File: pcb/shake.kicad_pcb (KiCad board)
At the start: 2 copper layers, 22.4 x 41.9 mm, 15 parts, among them T1 TO-92L_Inline

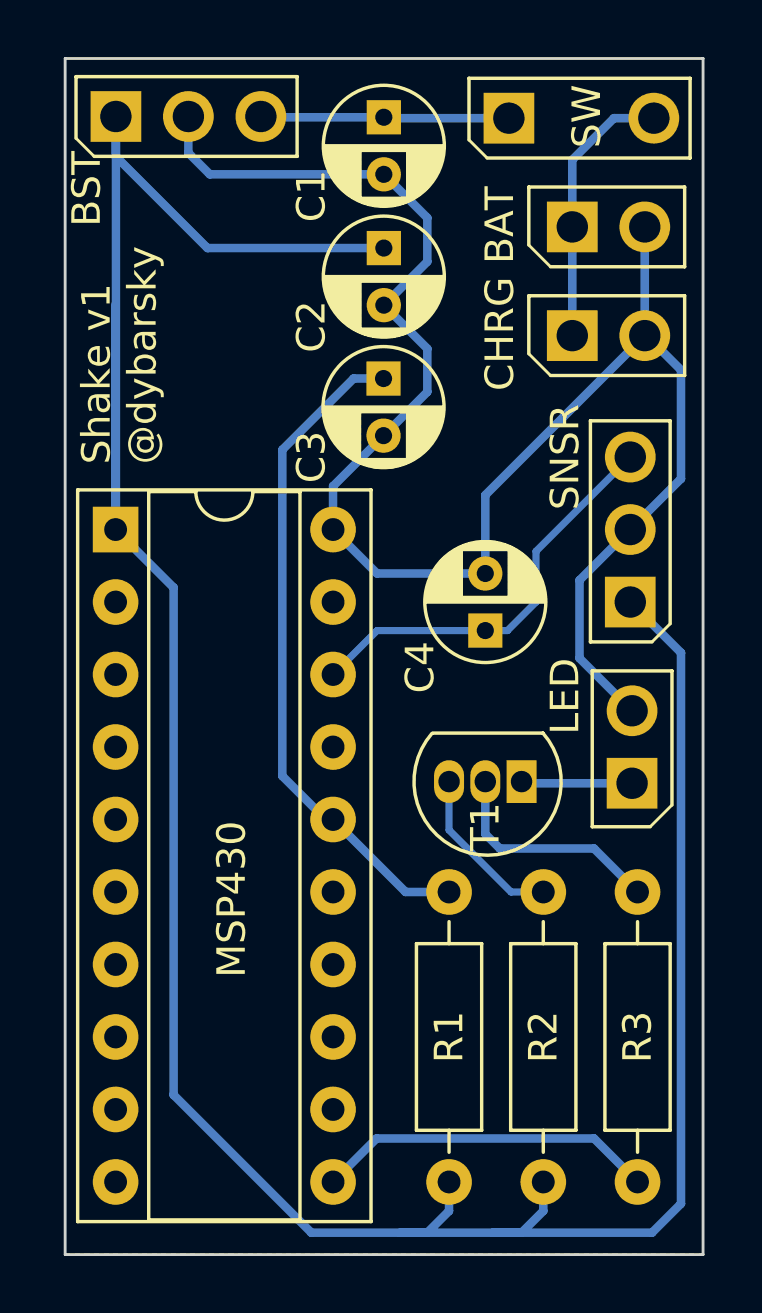
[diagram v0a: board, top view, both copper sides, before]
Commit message: Update kicad project
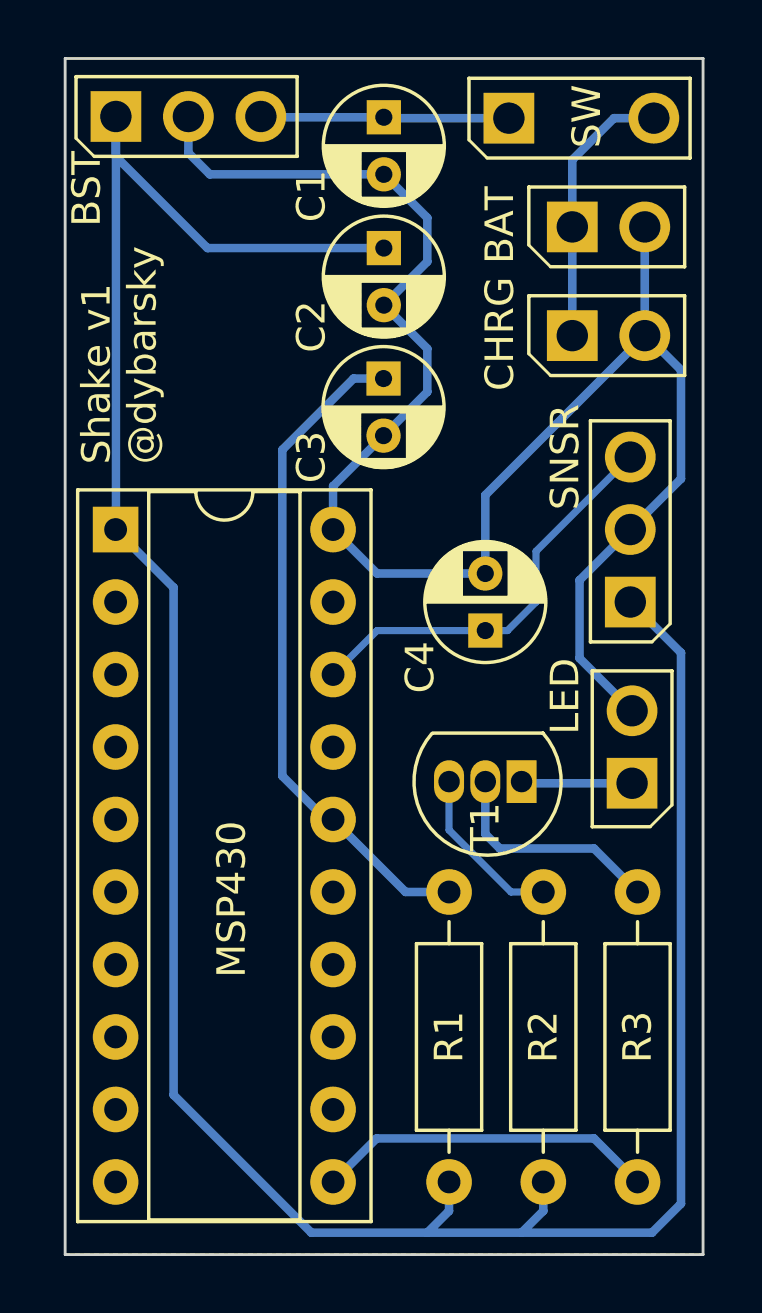
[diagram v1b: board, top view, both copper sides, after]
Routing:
- net +5V: track 110.5 -> 93.8 mm
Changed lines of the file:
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@@
     (grid_origin 85.08 69.591)
     (pcbplotparams
-      (layerselection 0x00010fc_ffffffff)
+      (layerselection 0x0001000_fffffffe)
       (plot_on_all_layers_selection 0x0000000_00000000)
       (disableapertmacros false)
@@
       (sketchpadsonfab false)
       (subtractmaskfromsilk false)
-      (outputformat 1)
+      (outputformat 5)
       (mirror false)
-      (drillshape 1)
+      (drillshape 2)
       (scaleselection 1)
       (outputdirectory "")
@@
   (segment (start 74.92 65.527) (end 74.92 61.717) (width 0.3) (layer "B.Cu") (net 3))
   (segment (start 55.118 67.564) (end 55.372 67.818) (width 0.3) (layer "F.Cu") (net 4))
-  (segment (start 55.108 59.431) (end 55.108 67.305) (width 0.3) (layer "B.Cu") (net 4))
   (segment (start 58.326401 57.442401) (end 55.118 54.234) (width 0.3) (layer "B.Cu") (net 4))
   (segment (start 55.118 52.832) (end 55.118 67.295) (width 0.3) (layer "B.Cu") (net 4))
   (segment (start 55.118 67.295) (end 55.108 67.305) (width 0.3) (layer "B.Cu") (net 4))
   (segment (start 73.904 91.943) (end 61.966 91.943) (width 0.3) (layer "B.Cu") (net 4))
-  (segment (start 69.332 91.943) (end 68.316 91.943) (width 0.3) (layer "B.Cu") (net 4))
-  (segment (start 66.03 91.943) (end 65.0775 91.943) (width 0.3) (layer "B.Cu") (net 4))
   (segment (start 64.506 57.442401) (end 58.326401 57.442401) (width 0.3) (layer "B.Cu") (net 4))
   (segment (start 57.14 87.117) (end 57.14 69.337) (width 0.3) (layer "B.Cu") (net 4))
@@
   (segment (start 66.792 91.181) (end 66.03 91.943) (width 0.3) (layer "B.Cu") (net 4))
   (segment (start 55.118 54.234) (end 55.118 52.832) (width 0.3) (layer "B.Cu") (net 4))
-  (segment (start 55.108 60.447) (end 55.108 67.305) (width 0.3) (layer "B.Cu") (net 4))
   (segment (start 70.094 90.165) (end 70.094 91.181) (width 0.3) (layer "B.Cu") (net 4))
   (segment (start 73.142 69.845) (end 74.92 71.623) (width 0.3) (layer "B.Cu") (net 4))

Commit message: Update pcb and schematics
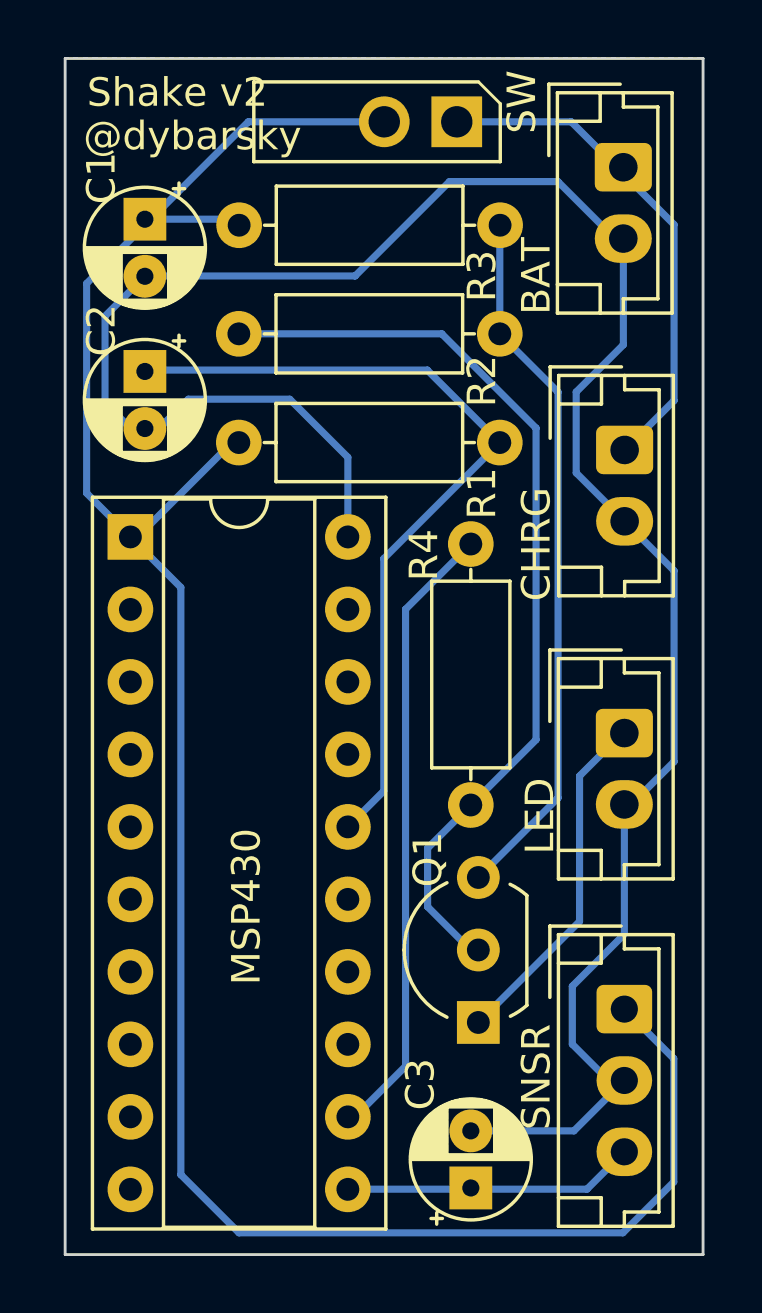
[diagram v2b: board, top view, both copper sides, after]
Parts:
- removed the BAT at (71.1, 56.7)
- removed BST: TerminalBlock_TE_282834-2_1x02_P2.54mm_Horizontal, TerminalBlock_TE-Connectivity:TerminalBlock_TE_282834-2_1x02_P2.54mm_Horizontal
- removed C4: CP_Radial_D4.0mm_P2.00mm, Capacitor_THT:CP_Radial_D4.0mm_P2.00mm
- removed the CHRG at (71.1, 60.5)
- removed the LED at (73.2, 76.2)
- removed the SNSR at (73.1, 69.8)
- removed T1: TO-92L_Inline, Package_TO_SOT_THT:TO-92L_Inline
- added BAT: JST_EH_B2B-EH-A_1x02_P2.50mm_Vertical, Connector_JST:JST_EH_B2B-EH-A_1x02_P2.50mm_Vertical, F.Cu at (72.9, 54.6)
- added CHRG: JST_EH_B2B-EH-A_1x02_P2.50mm_Vertical, Connector_JST:JST_EH_B2B-EH-A_1x02_P2.50mm_Vertical, F.Cu at (72.9, 64.5)
- added LED: JST_EH_B2B-EH-A_1x02_P2.50mm_Vertical, Connector_JST:JST_EH_B2B-EH-A_1x02_P2.50mm_Vertical, F.Cu at (72.9, 74.4)
- added Q1: TO-92L_Inline_Wide, Package_TO_SOT_THT:TO-92L_Inline_Wide, F.Cu at (67.8, 84.6)
- added R4: R_Axial_DIN0207_L6.3mm_D2.5mm_P10.16mm_Horizontal, Resistor_THT:R_Axial_DIN0207_L6.3mm_D2.5mm_P10.16mm_Horizontal, F.Cu at (67.6, 67.3)
- added SNSR: JST_EH_B3B-EH-A_1x03_P2.50mm_Vertical, Connector_JST:JST_EH_B3B-EH-A_1x03_P2.50mm_Vertical, F.Cu at (72.9, 84.1)
- moved R3 36.5 mm to (58.9, 56.6), turned to 0 degrees
- moved R2 29.7 mm to (69.1, 60.4), turned to 180 degrees
- moved C3 28.5 mm to (67.6, 90.4), turned to 90 degrees
- moved R1 27.1 mm to (58.9, 64.3), turned to 0 degrees
- moved C2 9.42 mm to (56.1, 61.8)
- moved C1 9.10 mm to (56.1, 56.4)
- moved SW 1.83 mm to (67.1, 53.0), turned to 180 degrees
- moved MSP430 0.58 mm to (55.6, 67.6)
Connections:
- C2 pad 1: +5V -> reset
- C3 pad 1: reset -> sensor
- MSP430 pad 1: +5V -> +3.7V
- MSP430 pad 11: led -> sensor
- MSP430 pad 12: (no net) -> led
- MSP430 pad 18: sensor -> (no net)
- R1 pad 1: +5V -> +3.7V
- R2 pad 1: +5V -> T1VCC
- R2 pad 2: T1VCC -> T1base
- R3 pad 1: led -> +3.7V
- R3 pad 2: T1base -> T1VCC
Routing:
- net +5V: track 93.8 -> 0.00 mm
- net +3.7V: track 18.3 -> 96.5 mm
- net T1base: track 8.01 -> 31.8 mm
- net T1VCC: track 5.90 -> 24.1 mm
- net GND: track 60.5 -> 75.7 mm
- net led: track 11.9 -> 22.0 mm
- net LedVcc: track 3.75 -> 12.3 mm
- net reset: track 23.0 -> 29.1 mm
- net sensor: track 14.6 -> 10.2 mm
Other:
- board text added: "@dybarsky"
- board text added: "Shake v2"
- board text removed: "Shake v1 @dybarsky"
